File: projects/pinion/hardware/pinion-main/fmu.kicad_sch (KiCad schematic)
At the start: 0 parts

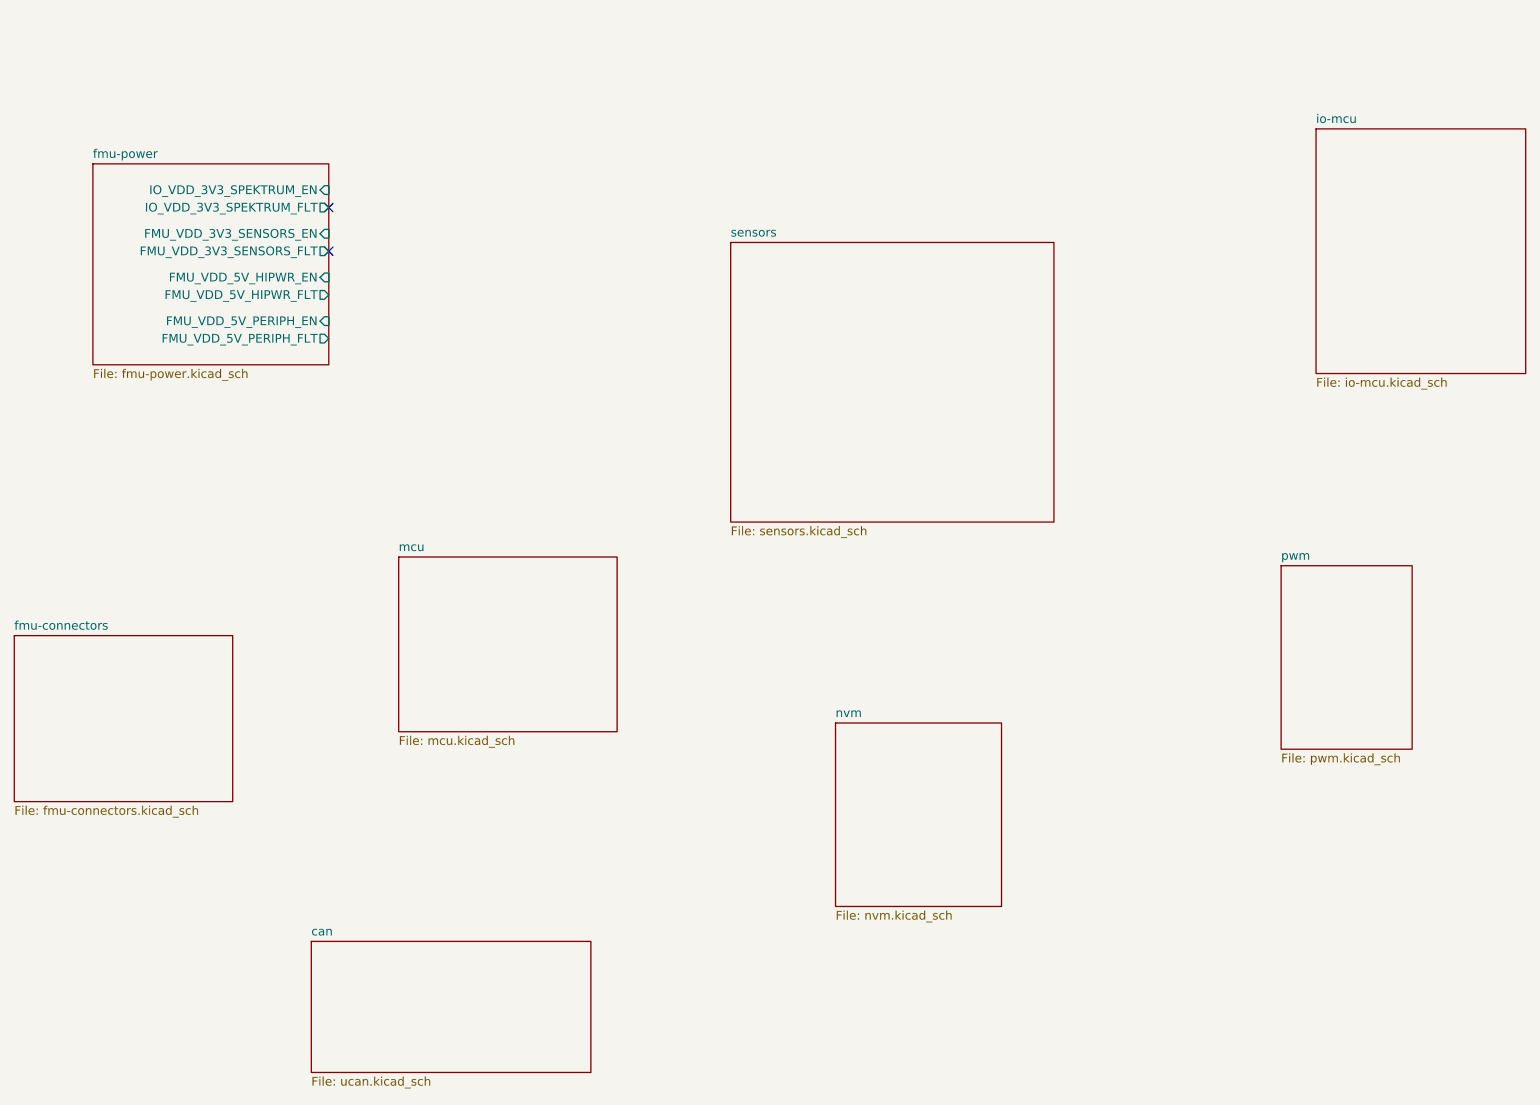
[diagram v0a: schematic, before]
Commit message: [pinion] fmu can transievers
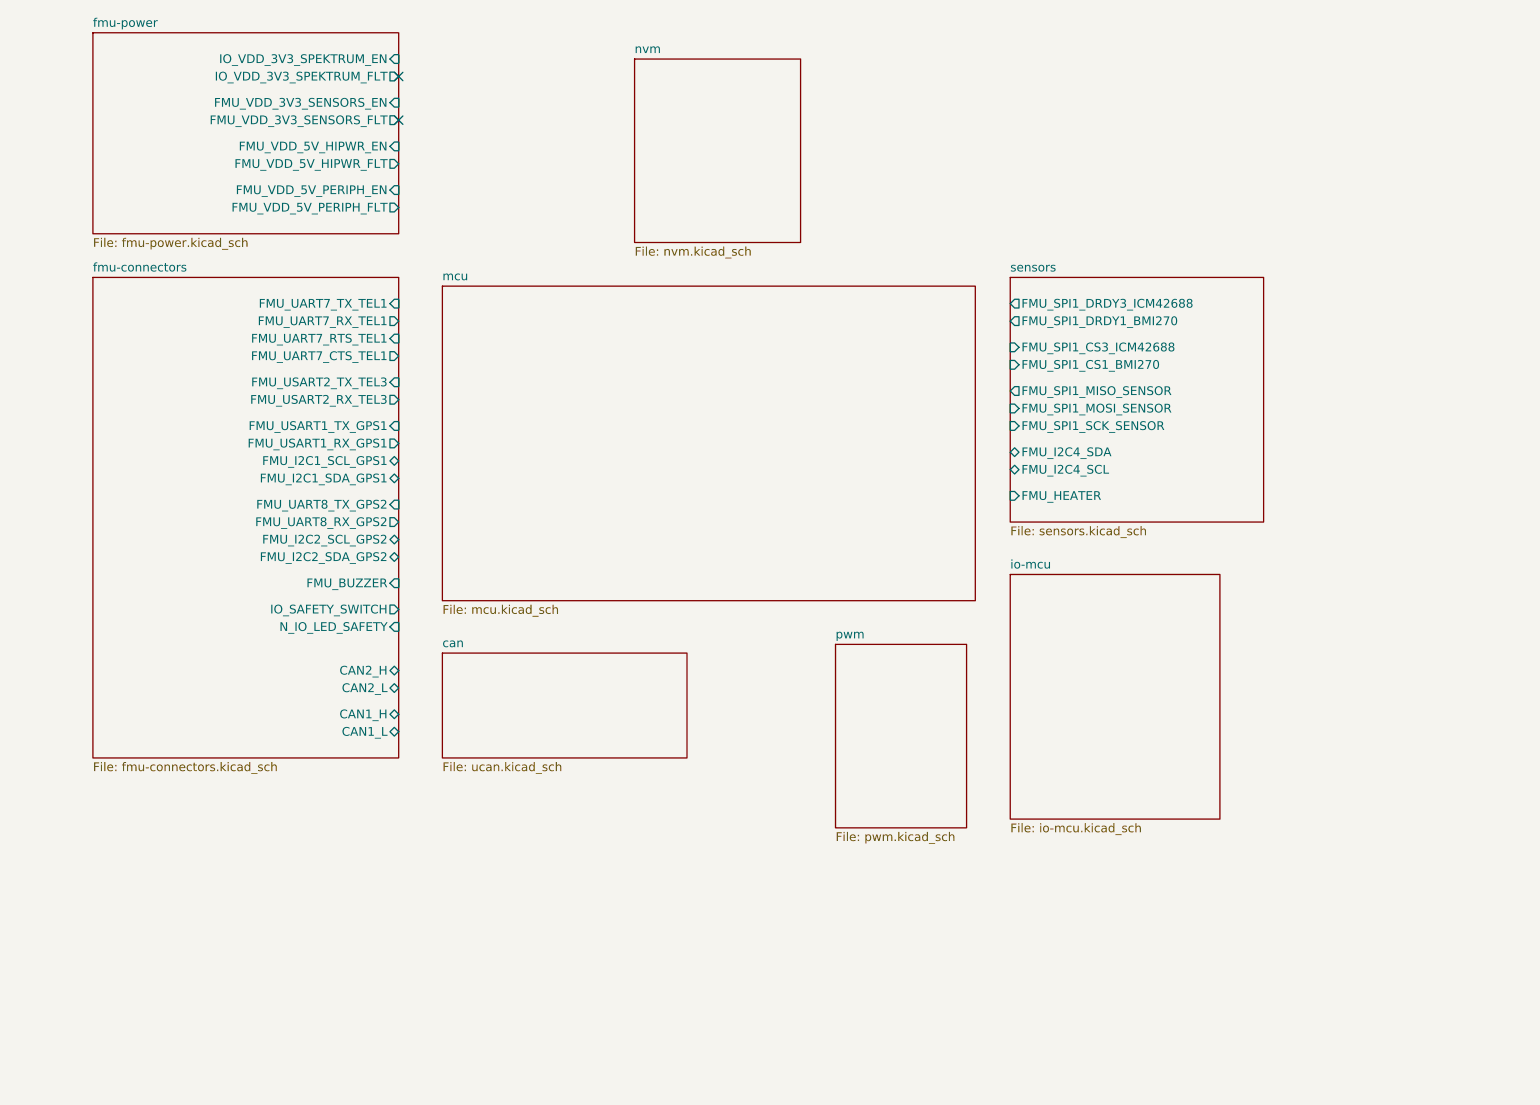
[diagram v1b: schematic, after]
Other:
- sheet fmu-connectors ports: added CAN1_H, CAN1_L, CAN2_H, CAN2_L, FMU_BUZZER, FMU_I2C1_SCL_GPS1, FMU_I2C1_SDA_GPS1, FMU_I2C2_SCL_GPS2, FMU_I2C2_SDA_GPS2, FMU_UART7_CTS_TEL1, FMU_UART7_RTS_TEL1, FMU_UART7_RX_TEL1, FMU_UART7_TX_TEL1, FMU_UART8_RX_GPS2, FMU_UART8_TX_GPS2, FMU_USART1_RX_GPS1, FMU_USART1_TX_GPS1, FMU_USART2_RX_TEL3, FMU_USART2_TX_TEL3, IO_SAFETY_SWITCH, N_IO_LED_SAFETY; removed none
- sheet sensors ports: added FMU_HEATER, FMU_I2C4_SCL, FMU_I2C4_SDA, FMU_SPI1_CS1_BMI270, FMU_SPI1_CS3_ICM42688, FMU_SPI1_DRDY1_BMI270, FMU_SPI1_DRDY3_ICM42688, FMU_SPI1_MISO_SENSOR, FMU_SPI1_MOSI_SENSOR, FMU_SPI1_SCK_SENSOR; removed none
